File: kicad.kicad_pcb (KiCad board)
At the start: 2 copper layers, 55.2 x 31.1 mm, 6 parts, among them J1 AKL059-03, J2 ESP8266, K1 JRC-21F(4100), U1 LD1117V33C_TO220

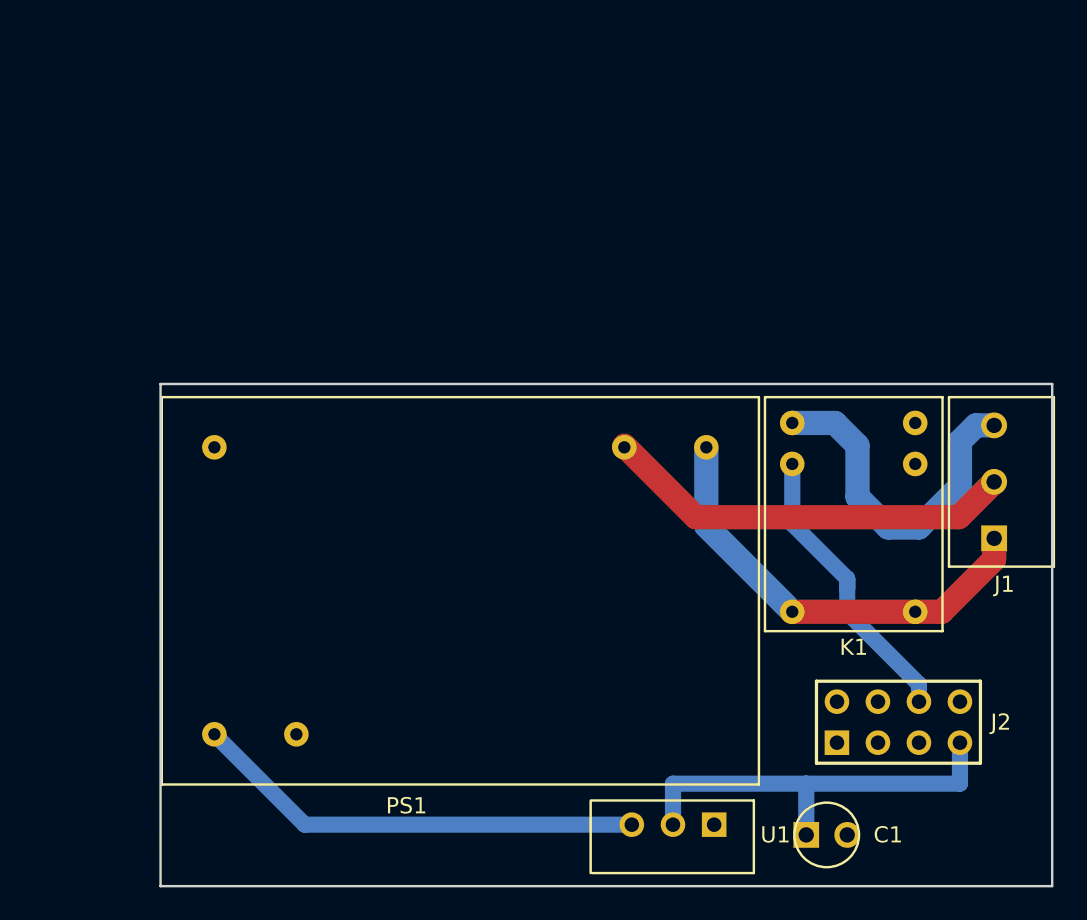
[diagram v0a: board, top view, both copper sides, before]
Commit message: v1.1
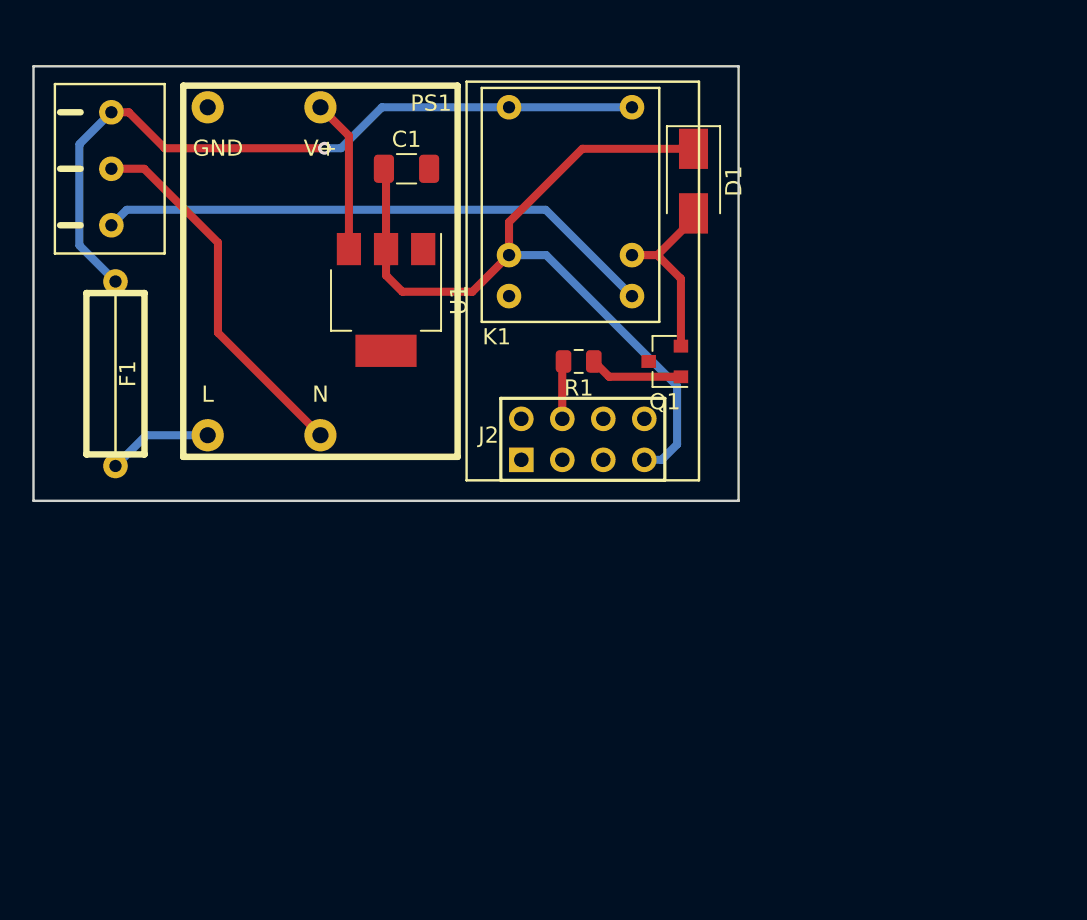
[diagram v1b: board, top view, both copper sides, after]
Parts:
- added D1: Diode, footprints:D_SMA, F.Cu at (153.7, 70.6)
- added F1: Fuse, footprints:Fuse, F.Cu at (117.9, 82.5)
- added G***: LOGO, footprints:logo, F.Cu at (105.2, 90.4)
- added G***: LOGO, footprints:logo, F.Cu at (102.9, 98.0)
- added Q1: MMBT4403, footprints:SOT-23, F.Cu at (151.9, 81.8)
- added R1: 1K, footprints:R_0805_2012Metric, F.Cu at (146.6, 81.8)
- C1: footprint footprints:C10uF -> footprints:C_1206_3216Metric
- J1: value AKL059-03 -> KF350; footprint footprints:AKL059-03 -> footprints:KF350
- PS1: value AC-12-3 -> 0102YN; footprint footprints:AC-12-3 -> footprints:0103YN
- U1: value LD1117V33C_TO220 -> LD1117V33C; footprint footprints:LD1117V33C-TO220 -> footprints:SOT-223
- moved J1 58.0 mm to (117.6, 69.8), turned to 270 degrees
- moved C1 48.8 mm to (135.9, 69.8)
- moved U1 37.1 mm to (134.6, 78.0), turned to 270 degrees
- moved J2 26.3 mm to (146.8, 86.6)
- moved K1 26.0 mm to (146.1, 72.1), turned to 270 degrees
- moved PS1 21.6 mm to (130.6, 76.2)
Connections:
- C1 pad 1: Net-(C1-Pad1) -> +3V3
- J1 pad 1: Net-(J1-Pad1) -> LINE
- J1 pad 2: +VSW -> Net-(J1-Pad2)
- J2 pad 3: Net-(C1-Pad1) -> Net-(J2-Pad3)
- J2 pad 4: Net-(J2-Pad4) -> +3V3
- J2 pad 7: GND -> Net-(J2-Pad7)
- K1 pad 1: GND -> LINE
- K1 pad 2: Net-(K1-Pad2) -> +3V3
- K1 pad 3: +VSW -> Net-(K1-Pad3)
- K1 pad 4: Net-(J2-Pad5) -> +VSW
- K1 pad 5: LINE -> Net-(D1-Pad2)
- PS1 pad 1: Net-(J1-Pad1) -> Net-(F1-Pad1)
- PS1 pad 2: Net-(PS1-Pad2) -> Net-(J1-Pad2)
- U1 pad 1: Net-(C1-Pad1) -> GND
- U1 pad 2: Net-(PS1-Pad3) -> +3V3
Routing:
- net +3V3: track 0.00 -> 50.8 mm
- net Net-(C1-Pad1): track 26.0 -> 0.00 mm
- net Net-(J1-Pad1): track 25.7 -> 0.00 mm
- net Net-(J1-Pad2): track 0.00 -> 23.1 mm
- net LINE: track 27.6 -> 46.5 mm, vias 0 -> 1
- net Net-(PS1-Pad3): track 28.2 -> 9.52 mm
- net Net-(J2-Pad5): track 18.6 -> 0.00 mm
- net +VSW: track 21.3 -> 34.9 mm
- net Net-(D1-Pad2): track 0.00 -> 11.3 mm
- net Net-(F1-Pad1): track 0.00 -> 6.50 mm
- net Net-(Q1-Pad2): track 0.00 -> 5.79 mm
- net Net-(J2-Pad7): track 0.00 -> 3.59 mm
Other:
- board size 55.2 x 31.1 mm -> 43.7 x 26.9 mm
- board text removed: "3V3"
- board text removed: "EN"
- board text removed: "GND"
- board text removed: "I00"
- board text removed: "I02"
- board text removed: "IN"
- board text removed: "OUT"
- board text removed: "RST"
- board text removed: "RX"
- board text removed: "TX"
- board text removed: "V+"
- board text removed: "V-"

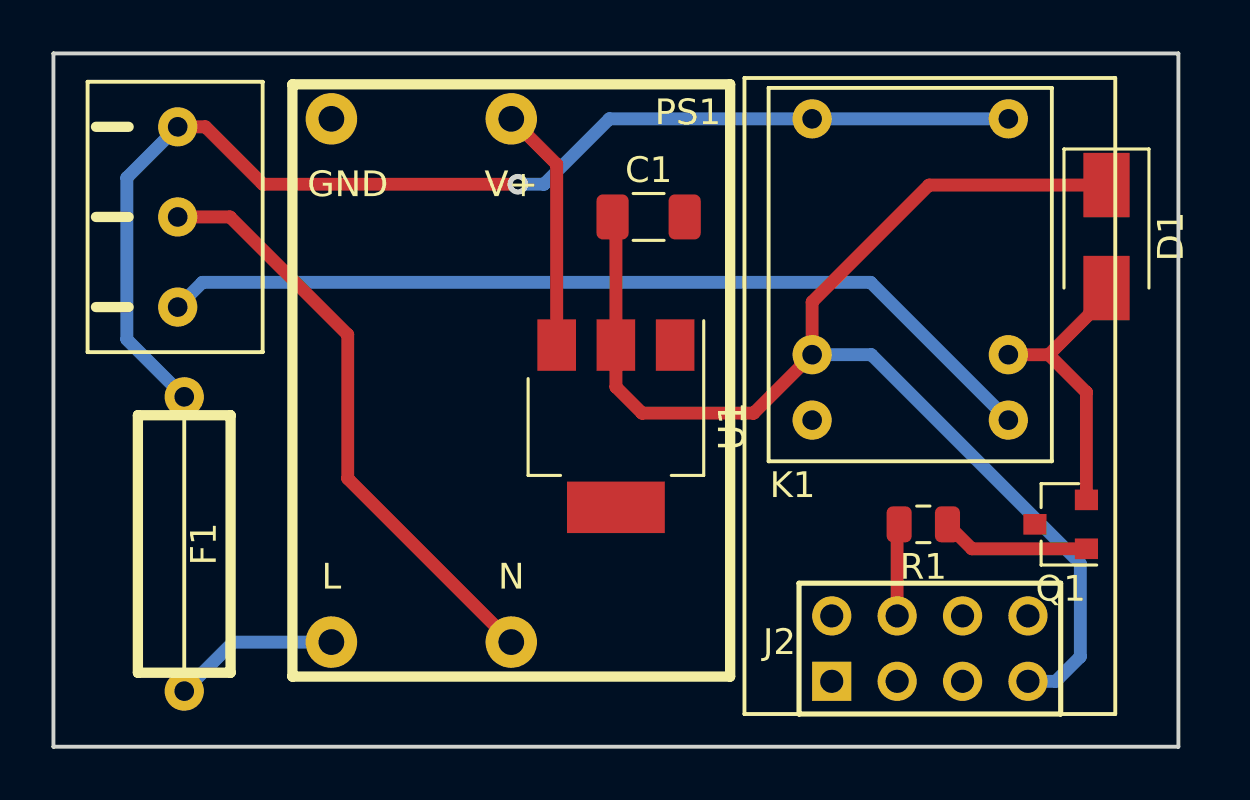
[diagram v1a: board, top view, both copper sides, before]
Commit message: Update version 1.1
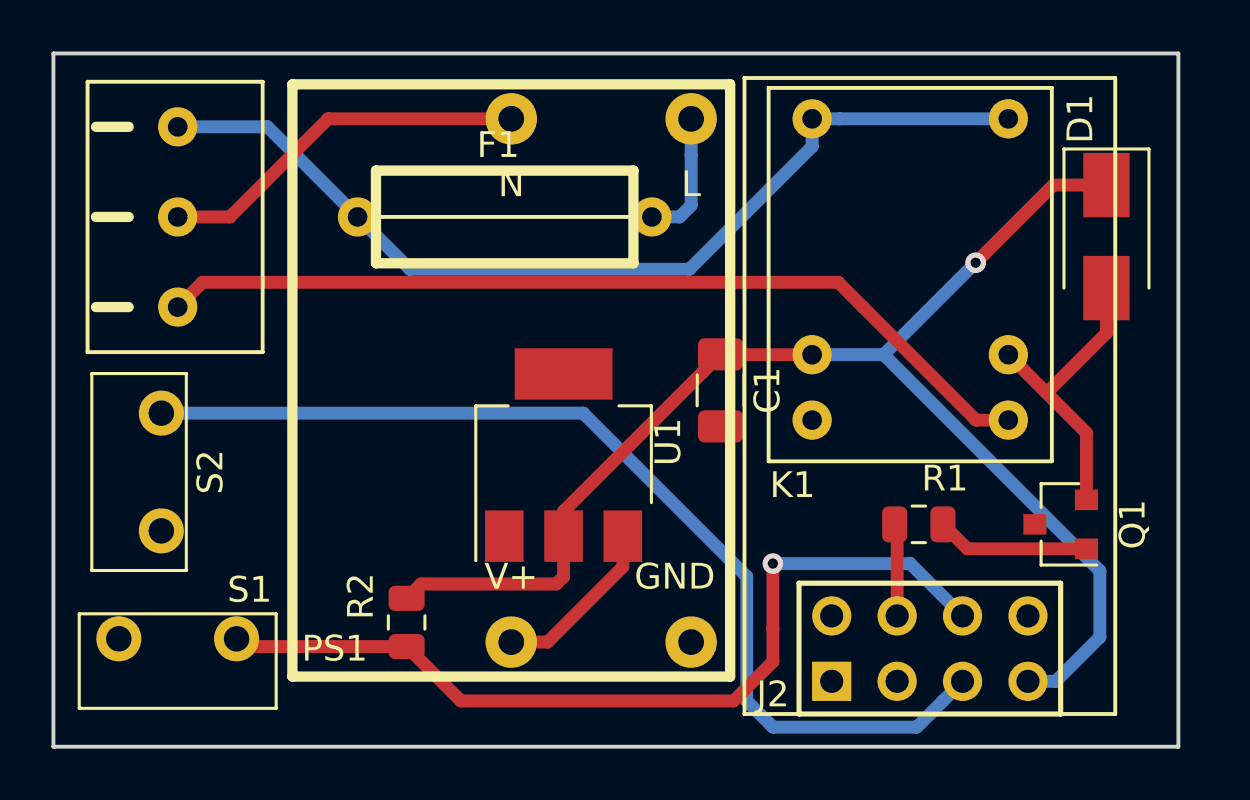
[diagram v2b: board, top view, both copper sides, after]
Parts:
- added G***: LOGO, footprints:logo, B.Cu at (136.9, 74.7)
- added R2: 10K, footprints:R_0805_2012Metric, F.Cu at (126.5, 85.6)
- added S1: init setup, footprints:SW_Tactile, F.Cu at (117.6, 87.1)
- added S2: reset, footprints:SW_Tactile, F.Cu at (116.1, 79.8)
- moved F1 17.8 mm to (130.3, 69.8), turned to 180 degrees
- moved C1 7.29 mm to (138.7, 76.6), turned to 270 degrees
- moved U1 2.32 mm to (132.6, 79.1), turned to 90 degrees
- moved R1 0.18 mm to (146.4, 81.8)
- turned PS1 to 180 degrees
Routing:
- net Net-(J2-Pad3): track 0.00 -> 39.7 mm
- net Net-(J2-Pad6): track 0.00 -> 34.5 mm, vias 0 -> 1
- net LINE: track 46.5 -> 37.6 mm, vias 1 -> 0
- net Net-(J1-Pad2): track 23.1 -> 14.5 mm
- net Net-(PS1-Pad3): track 9.52 -> 6.74 mm
- net +3V3: track 50.8 -> 53.3 mm, vias 0 -> 1
- net Net-(F1-Pad1): track 6.50 -> 5.07 mm
- net Net-(D1-Pad2): track 11.3 -> 11.9 mm
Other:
- board text added: "Smart home V1.1"

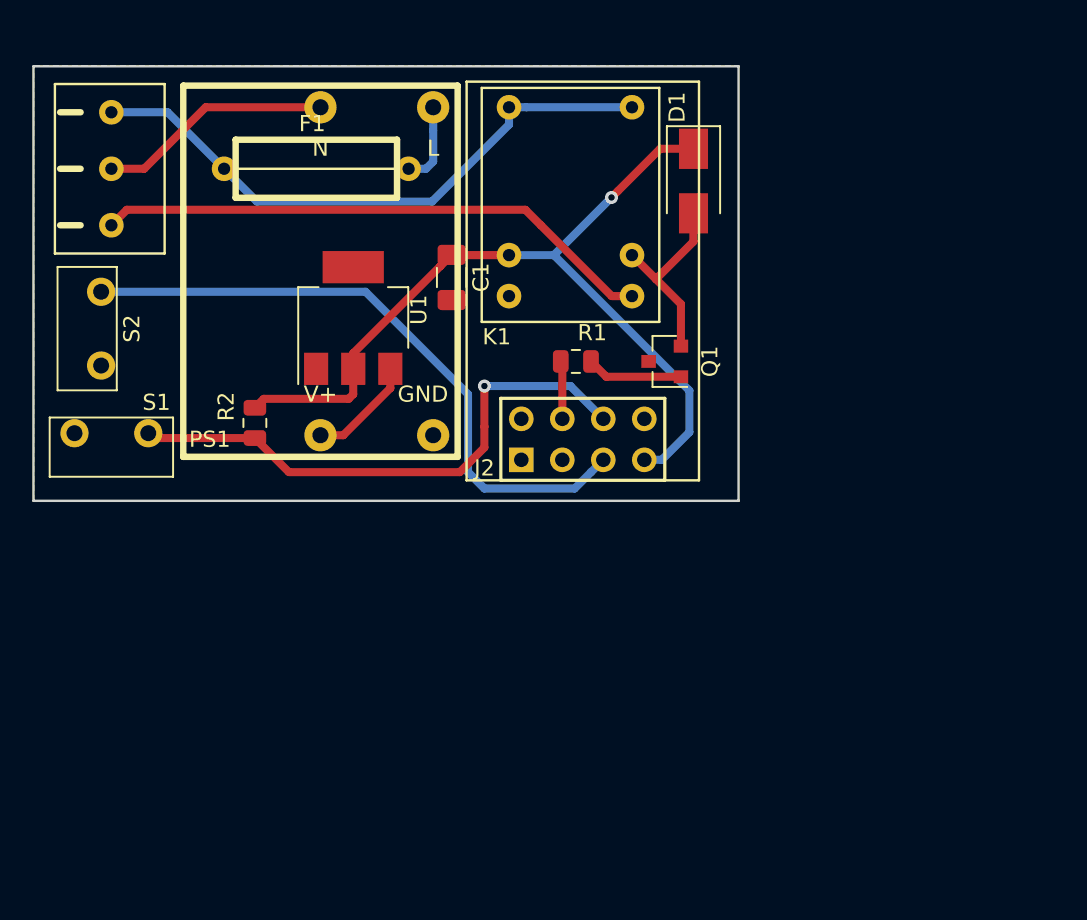
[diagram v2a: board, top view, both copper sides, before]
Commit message: Version 1.2
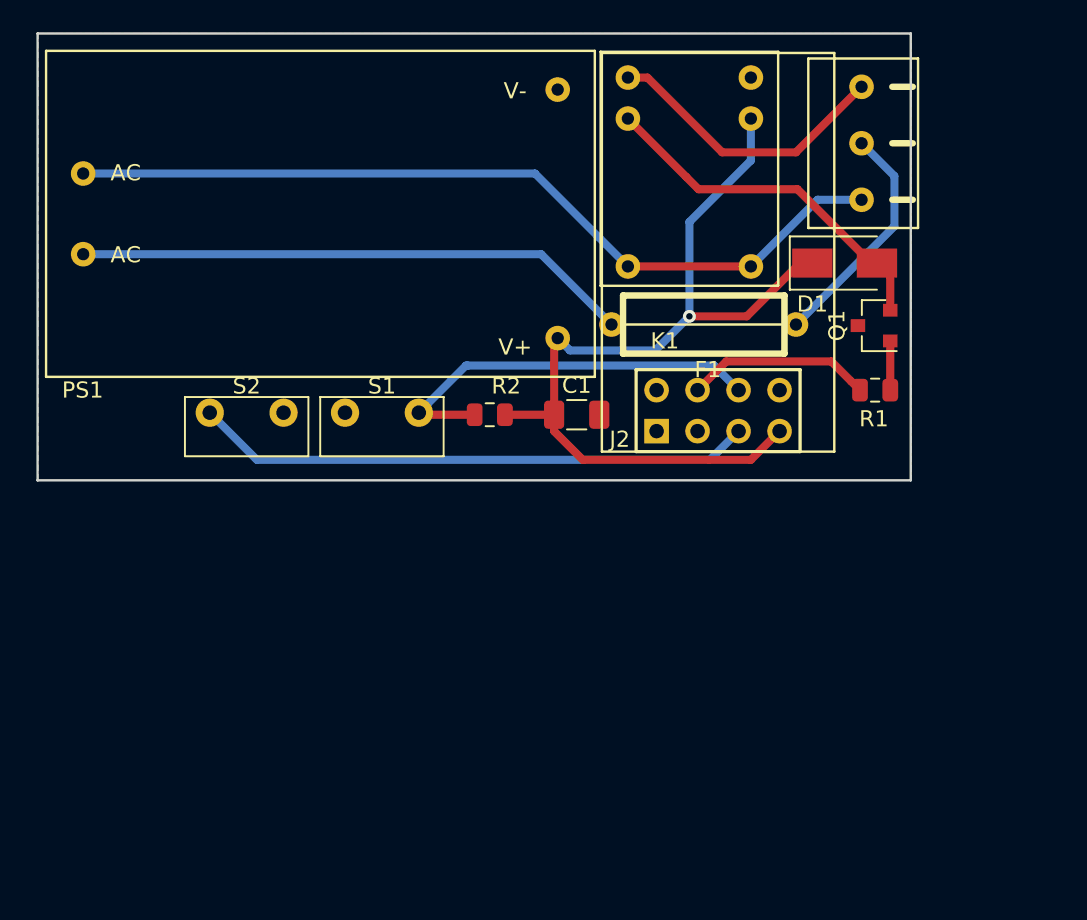
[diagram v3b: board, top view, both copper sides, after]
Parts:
- removed U1: LD1117V33C, footprints:SOT-223
- PS1: value 0102YN -> HLK-PM; footprint footprints:0103YN -> footprints:HLK-PM
- moved J1 46.5 mm to (164.1, 68.3), turned to 90 degrees
- moved F1 25.9 mm to (154.3, 79.5), turned to 0 degrees
- moved R1 18.6 mm to (164.9, 83.6)
- moved S1 16.8 mm to (134.4, 85.9)
- moved R2 14.6 mm to (141.0, 85.1), turned to 0 degrees
- moved Q1 13.2 mm to (164.9, 79.6)
- moved S2 11.6 mm to (126.0, 85.9), turned to 180 degrees
- moved C1 11.5 mm to (146.4, 85.1), turned to 0 degrees
- moved D1 10.7 mm to (163.0, 75.7), turned to 0 degrees
- moved J2 8.57 mm to (155.2, 84.8)
- moved K1 7.70 mm to (153.4, 69.8), turned to 90 degrees
- moved PS1 3.56 mm to (130.6, 72.6), turned to 0 degrees
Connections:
- F1 pad 2: LINE -> Net-(F1-Pad2)
- J1 pad 2: Net-(J1-Pad2) -> Net-(F1-Pad2)
- PS1 pad 1: Net-(F1-Pad1) -> LINE
- PS1 pad 2: Net-(J1-Pad2) -> Net-(F1-Pad1)
- PS1 pad 3: Net-(PS1-Pad3) -> GND
- PS1 pad 4: GND -> +3V3
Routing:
- net Net-(F1-Pad1): track 5.07 -> 34.5 mm
- net +VSW: track 34.9 -> 18.1 mm
- net LINE: track 37.6 -> 52.3 mm
- net Net-(F1-Pad2): track 0.00 -> 14.6 mm
- net Net-(J1-Pad2): track 14.5 -> 0.00 mm
- net Net-(D1-Pad2): track 11.9 -> 22.4 mm
- net Net-(J2-Pad6): track 34.5 -> 25.2 mm, vias 1 -> 0
- net Net-(J2-Pad7): track 3.60 -> 11.5 mm
- net Net-(PS1-Pad3): track 6.74 -> 0.00 mm
- net Net-(J2-Pad3): track 39.7 -> 34.7 mm
- net +3V3: track 53.3 -> 56.8 mm
- net Net-(Q1-Pad2): track 5.97 -> 3.05 mm
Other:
- board size 43.7 x 26.9 mm -> 54.1 x 27.7 mm
- board text added: "Smart home V1.2"
- board text removed: "Smart home V1.1"
